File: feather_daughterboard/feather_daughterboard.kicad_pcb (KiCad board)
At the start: 2 copper layers, 79.7 x 11 mm, 20 parts, among them J1 6250XX21721_62501021721

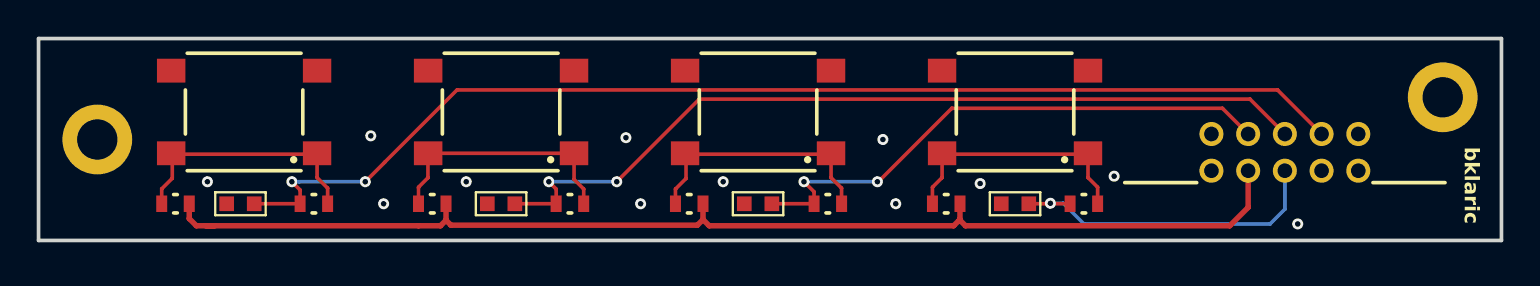
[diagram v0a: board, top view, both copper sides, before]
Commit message: finished mainboard and daughterboard
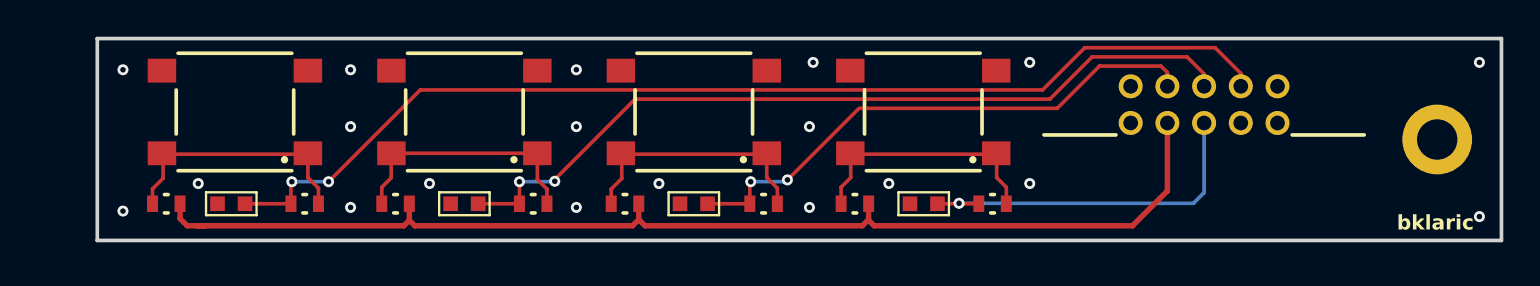
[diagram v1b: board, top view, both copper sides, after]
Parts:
- removed H2: MountingHole_Pad, MountingHole:MountingHole_2.2mm_M2_DIN965_Pad
- moved J1 5.11 mm to (168.8, 87.2)
- moved S1 5.00 mm to (153.5, 83.0)
- moved C1_1 4.98 mm to (153.5, 88.0)
- moved R1_1 4.98 mm to (157.3, 88.0)
- moved R2_1 4.98 mm to (149.8, 88.0)
- moved C1_2 3.50 mm to (141.0, 88.0)
- moved R1_2 3.50 mm to (144.8, 88.0)
- moved R2_2 3.50 mm to (137.2, 88.0)
- moved S2 3.50 mm to (141.0, 83.0)
- moved H1 2.32 mm to (181.5, 84.5)
- moved C1_3 2.00 mm to (128.5, 88.0)
- moved R1_3 2.00 mm to (132.2, 88.0)
- moved R2_3 2.00 mm to (124.8, 88.0)
- moved S3 2.00 mm to (128.5, 83.0)
- moved G*** 1.63 mm to (116.6, 85.3)
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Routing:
- net /Buttons/Button_4: track 63.1 -> 59.8 mm
- net /Buttons/VCC: track 65.4 -> 63.2 mm
- net /Buttons/Button_1: track 18.0 -> 19.7 mm
- net /Buttons/Button_3: track 46.4 -> 44.7 mm
- net /Buttons/GND: vias 12 -> 19
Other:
- board size 79.7 x 11 mm -> 76.5 x 11 mm
